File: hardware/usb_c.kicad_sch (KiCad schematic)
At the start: 22 parts, among them Q1 SS8050_C2150, Q2 SS8050_C2150, U2 CH343G

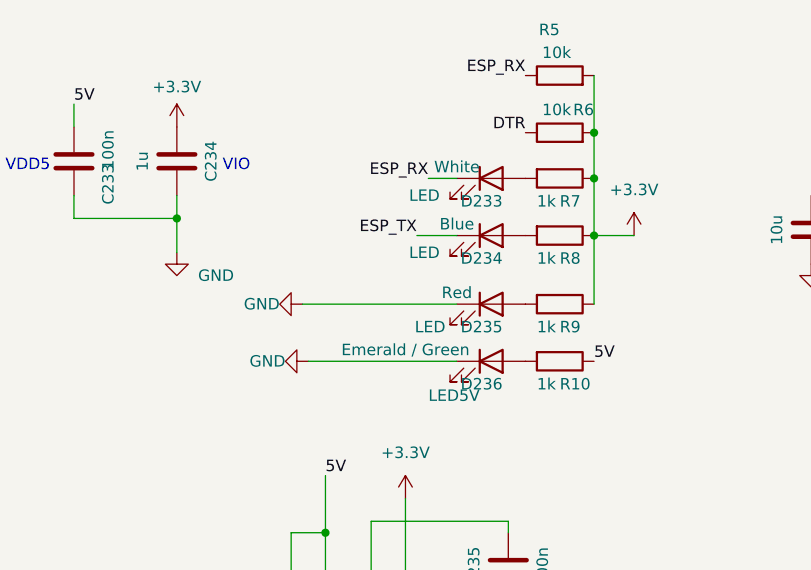
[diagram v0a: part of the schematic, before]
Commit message: PCB rework (ordered)
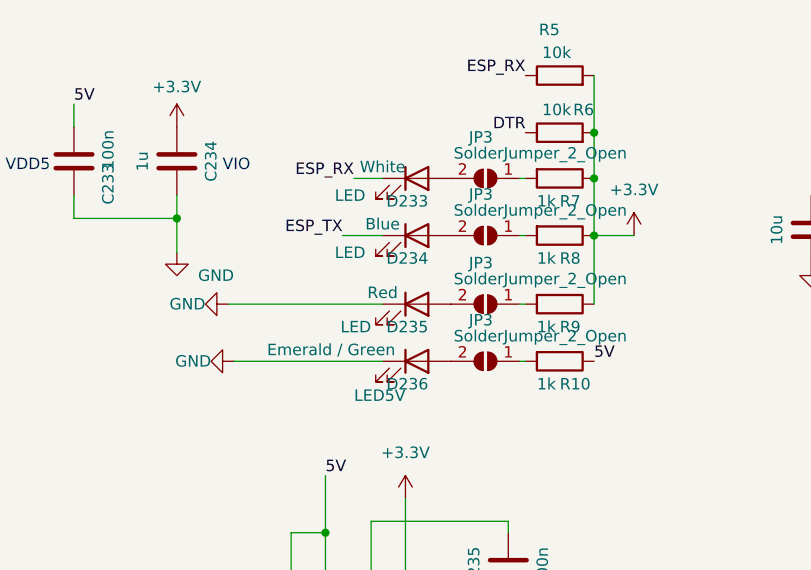
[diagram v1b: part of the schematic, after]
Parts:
- added JP3 (x4): SolderJumper_2_Open, Jumper:SolderJumper-2_P1.3mm_Open_TrianglePad1.0x1.5mm, symbol Jumper:SolderJumper_2_Open
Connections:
- net at R8.2: now also JP3.1 (A); no longer D234.2 (A)
- net at D235.2 (A): now also JP3.2 (B); no longer R9.2
- net at R10.2: now also JP3.1 (A); no longer D236.2 (A)
- net at R7.2: now also JP3.1 (A); no longer D233.2 (A)
- new net: D236.2 (A), JP3.2 (B)
- new net: D234.2 (A), JP3.2 (B)
- new net: JP3.1 (A), R9.2
- new net: D233.2 (A), JP3.2 (B)
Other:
- moved on the sheet: D233, D234, D235, D236
